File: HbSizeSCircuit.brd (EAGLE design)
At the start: 38.8 x 45.9 mm, 20 parts

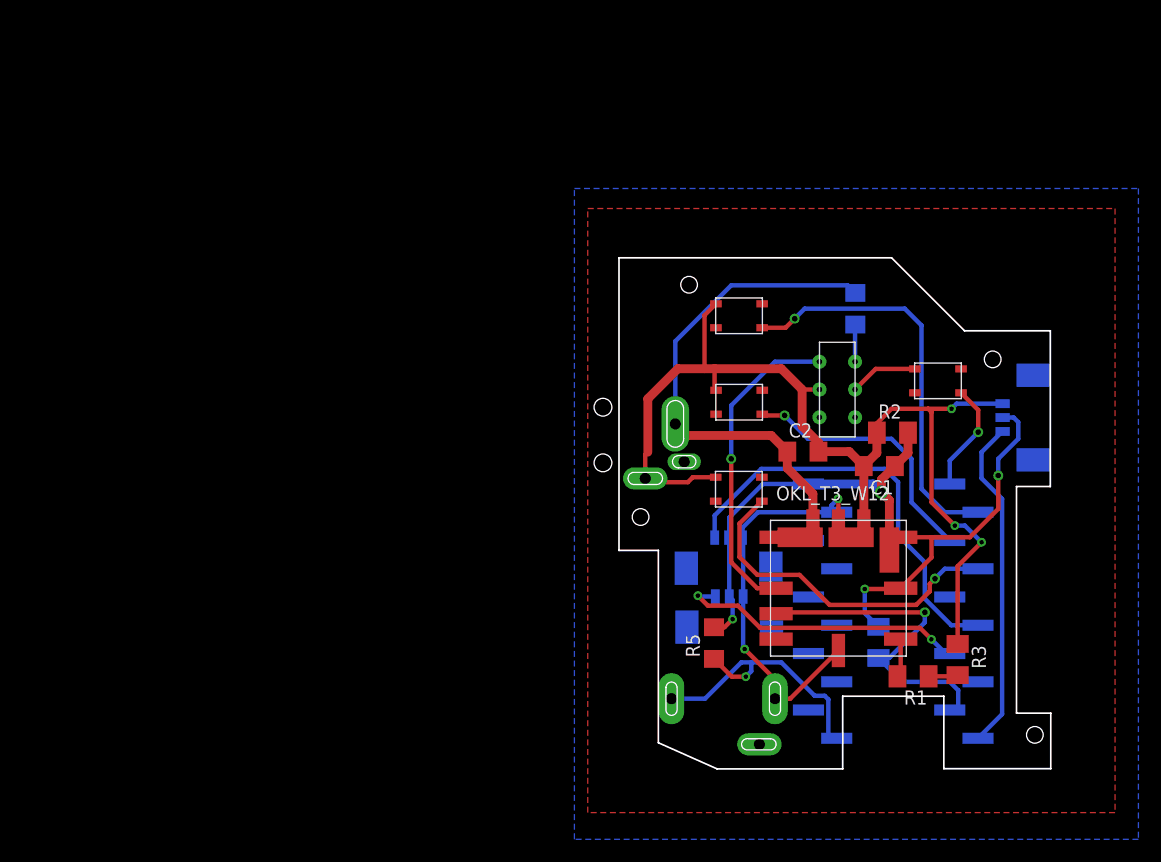
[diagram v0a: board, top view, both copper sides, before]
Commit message: add left board file
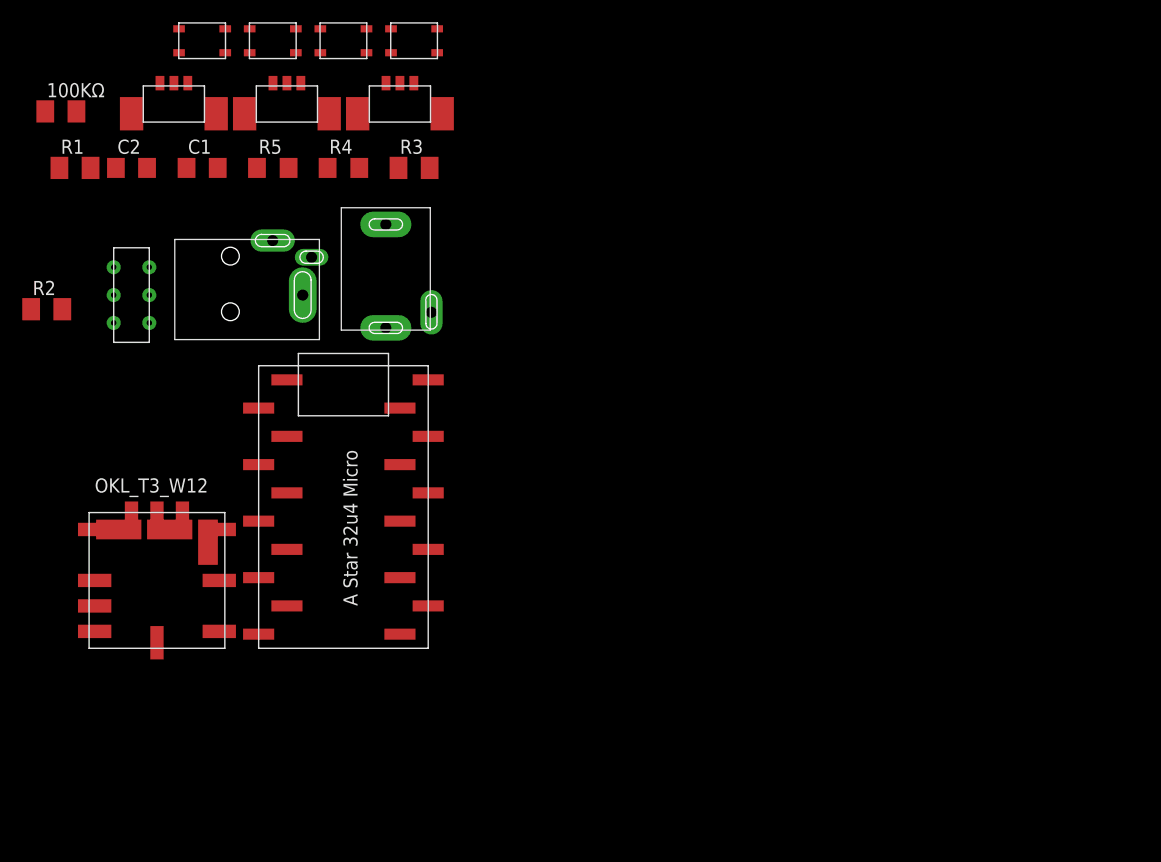
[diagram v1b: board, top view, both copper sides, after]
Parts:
- moved R1 88.1 mm to (-47.0, 44.5), turned to 0 degrees
- moved 100KΩ 87.6 mm to (-48.3, 49.5), flipped to the top, turned to 0 degrees
- moved U$12 80.3 mm to (-38.1, 52.1), flipped to the top, turned to 0 degrees
- moved R2 76.8 mm to (-49.5, 31.8)
- moved U$5 72.9 mm to (-35.6, 55.9)
- moved C1 66.5 mm to (-35.6, 44.5), turned to 0 degrees
- moved R3 65.9 mm to (-16.5, 44.5), turned to 0 degrees
- moved C2 65.5 mm to (-41.9, 44.5)
- moved U$2 64.0 mm to (-41.9, 33.0)
- moved U$8 61.3 mm to (-45.7, 1.27)
- moved U$11 60.9 mm to (-27.9, 52.1), flipped to the top
- moved R5 58.3 mm to (-29.2, 44.5), turned to 0 degrees
- moved U$4 58.1 mm to (-29.2, 55.9)
- moved U$9 50.4 mm to (-17.8, 52.1), flipped to the top
- moved U$6 50.3 mm to (-22.9, 14.0), flipped to the top, turned to 0 degrees
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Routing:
- net GND: track 142.9 -> 0.00 mm, vias 5 -> 0
- net +5V: track 72.8 -> 0.00 mm, vias 4 -> 0
- net V+: track 48.4 -> 0.00 mm
- net PIN_THUMBSERVO: track 38.0 -> 0.00 mm
- net SWITCH_INIT: track 36.3 -> 0.00 mm, vias 1 -> 0
- net PIN_ON/OFF: track 32.0 -> 0.00 mm, vias 1 -> 0
- net SWITCH_THUMB: track 30.8 -> 0.00 mm, vias 1 -> 0
- net PIN_INDEXSERVO: track 30.0 -> 0.00 mm
- net PGOOD: track 30.0 -> 0.00 mm, vias 1 -> 0
- net PIN_OTHERSERVO: track 26.4 -> 0.00 mm, vias 2 -> 0
- net SENSOR: track 25.3 -> 0.00 mm, vias 1 -> 0
- net SWITCH_MODE: track 23.8 -> 0.00 mm, vias 1 -> 0
- net SWITCH_HOLD: track 9.90 -> 0.00 mm, vias 1 -> 0
- net N$1: track 3.46 -> 0.00 mm
- net N$2: track 2.66 -> 0.00 mm
- removed copper zone on layer 1, net GND
- removed copper zone on layer 16, net GND
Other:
- board size 38.8 x 45.9 mm -> 6.1 x 10.3 mm
